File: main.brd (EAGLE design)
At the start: 74.6 x 58.4 mm, 25 parts, among them IC1 SN754410, IC2 7805T, T1 BPX81, T2 BPX81, T3 BPX81, T4 BPX81

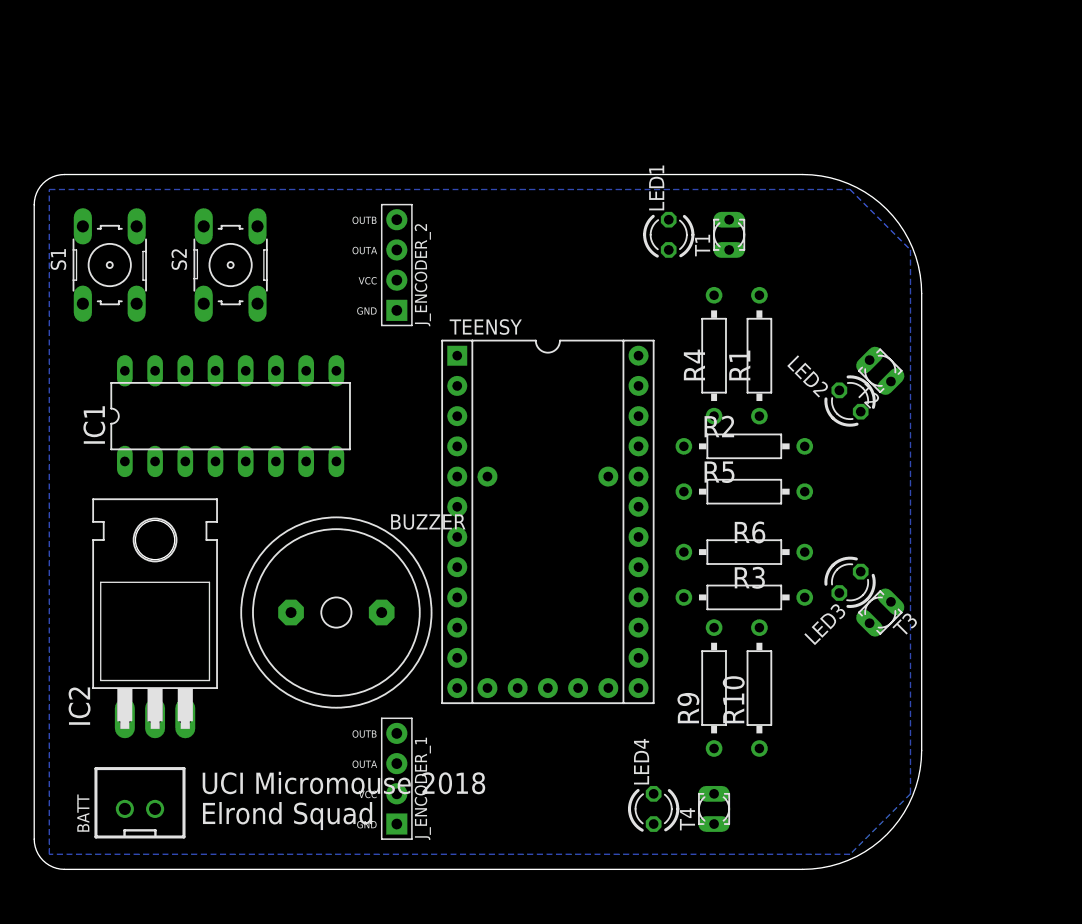
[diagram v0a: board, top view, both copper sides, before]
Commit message: Peer Review Version
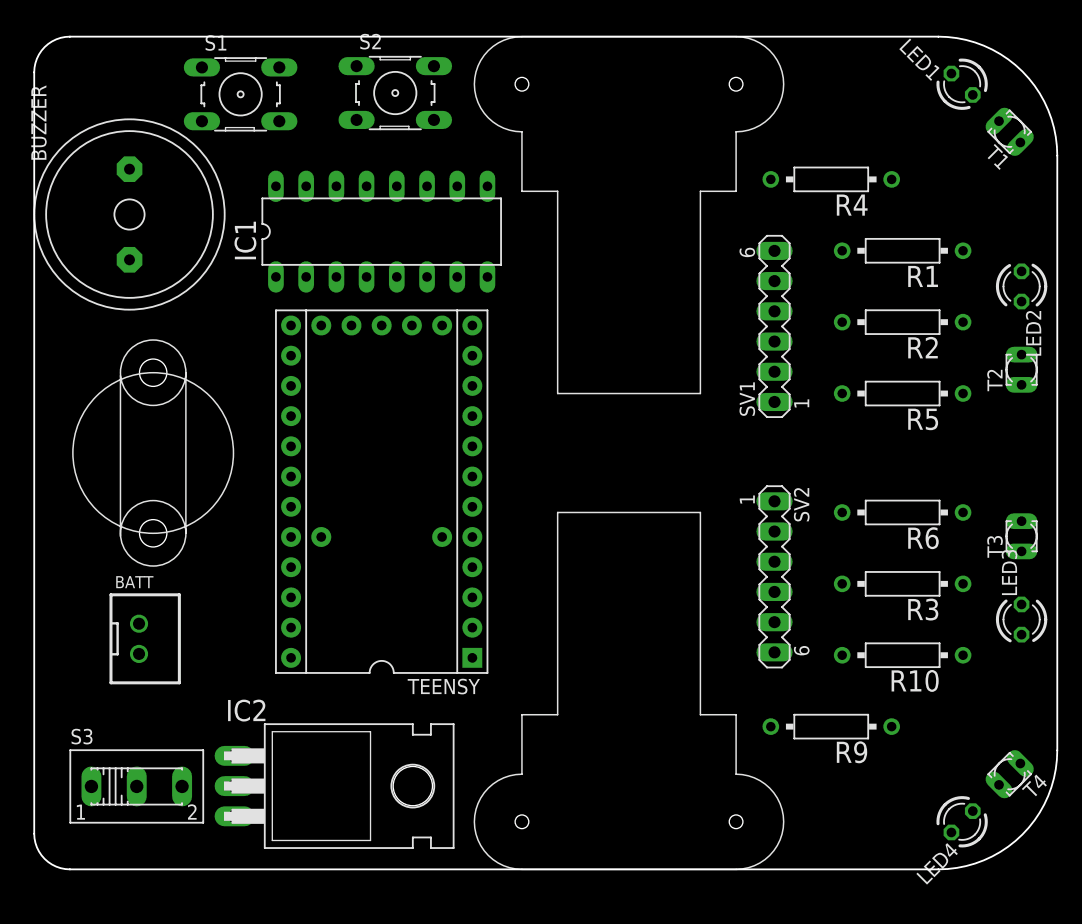
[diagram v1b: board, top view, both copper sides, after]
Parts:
- removed J_ENCODER_1, J_ENCODER_2: ENCODER, Pololu Encoder and Motor Driver:ENCODER_FOOTPRINT
- added S3: (no value), switch:255SB
- added SV1, SV2: (no value), con-lstb:MA06-1
- added U$1, U$2: POLULUMOTOR, personal:FP
- added U$3: CASTERBALL, personal:FB_CASTER
- moved BUZZER 37.7 mm to (8.01, 55.0), turned to 90 degrees
- moved LED1 27.7 mm to (78.0, 66.0), turned to 135 degrees
- moved LED4 26.0 mm to (78.0, 4.00), turned to 225 degrees
- moved T1 25.1 mm to (82.0, 62.0), turned to 135 degrees
- moved T4 25.0 mm to (82.0, 8.00), turned to 225 degrees
- moved IC2 23.1 mm to (27.0, 7.00), turned to 270 degrees
- moved IC1 20.0 mm to (30.5, 53.6)
- moved S2 20.0 mm to (30.4, 65.3), turned to 0 degrees
- moved S1 18.1 mm to (17.4, 65.2), turned to 0 degrees
- moved R4 17.8 mm to (67.0, 58.0), turned to 180 degrees
- moved LED2 17.3 mm to (83.0, 49.0), turned to 270 degrees
- moved R2 16.9 mm to (73.0, 46.0)
- moved R5 15.7 mm to (73.0, 40.0)
- moved R1 14.9 mm to (73.0, 52.0), turned to 180 degrees
- moved LED3 14.8 mm to (83.0, 21.0), turned to 90 degrees
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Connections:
- removed net L3: R6.2, TEENSY.B2
- removed net L4: R9.2, TEENSY.D1
- removed net N$2: IC1.3, J_ENCODER_1.OUTA
- removed net N$3: IC1.6, J_ENCODER_1.OUTB
- removed net N$4: IC1.11, J_ENCODER_2.OUTB
- removed net N$5: IC1.14, J_ENCODER_2.OUTA
- new net ENC1A: SV1.3, TEENSY.F7
- new net ENC1B: SV1.2, TEENSY.F6
- new net ENC2A: SV2.3, TEENSY.B2
- new net ENC2B: SV2.2, TEENSY.B6
- new net M1A: IC1.3, SV1.6
- new net M1B: IC1.6, SV1.5
- new net M2A: IC1.14, SV2.6
- new net M2B: IC1.11, SV2.5
- new net N$10: IC2.3, S3.2
- new net VM1: SV1.4
- new net VM2: SV2.4
- net +5V: now also S3.3; no longer IC2.3, J_ENCODER_1.VCC, J_ENCODER_2.VCC
- net GND: now also SV1.1, SV2.1; no longer J_ENCODER_1.GND, J_ENCODER_2.GND
- net L1: now also R9.2
- net L2: now also R6.2
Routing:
- removed copper zone on layer 16, net GND
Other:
- board size 74.6 x 58.4 mm -> 86 x 70 mm
- board text removed: "Elrond Squad"
- board text removed: "UCI Micromouse 2018"
